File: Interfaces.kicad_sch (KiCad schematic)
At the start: 17 parts, among them J3 Conn_01x04_MountingPin, J4 Conn_01x05_Pin, J5 Conn_01x05_MountingPin, J6 MSD-11-A, U5 TLV74033PDBVR

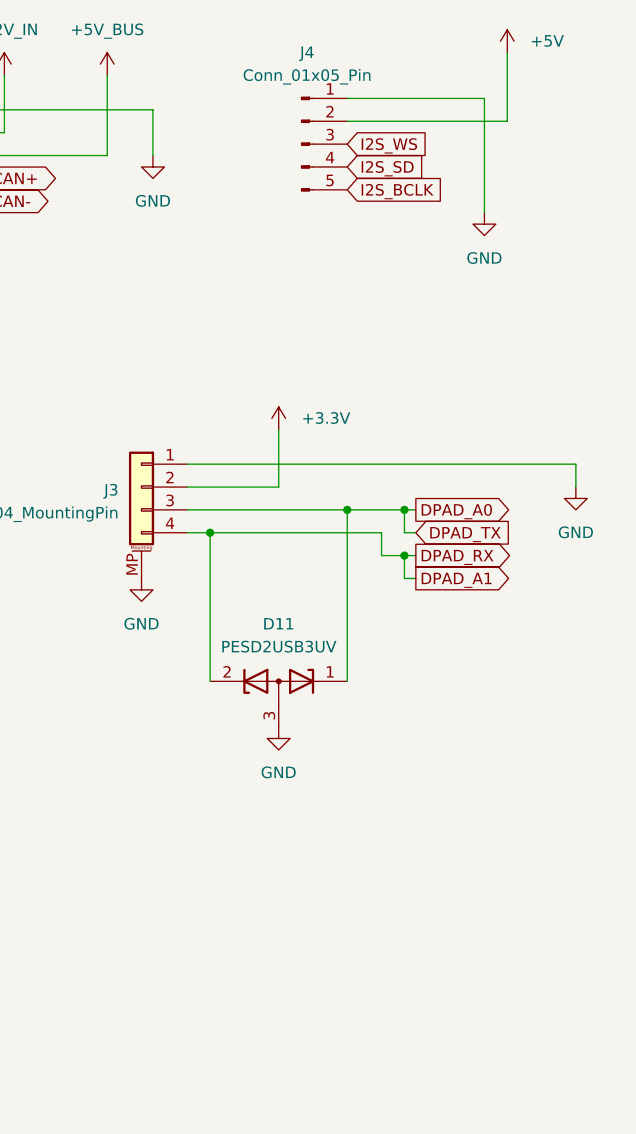
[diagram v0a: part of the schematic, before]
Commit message: r1 final (see changelog.md)
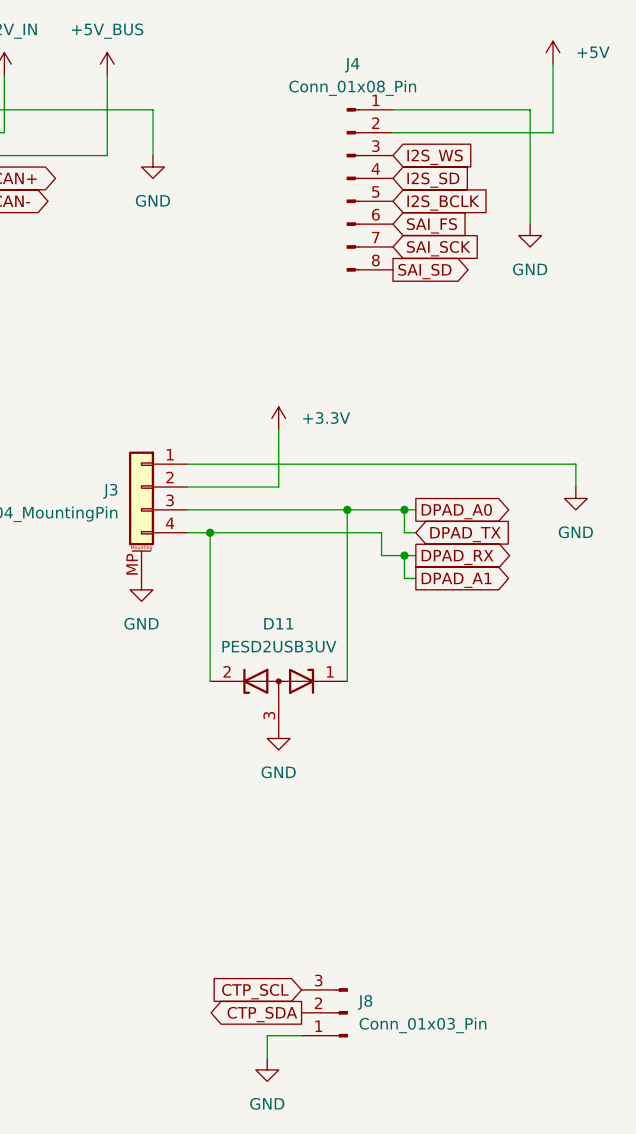
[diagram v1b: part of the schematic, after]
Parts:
- removed J4: Conn_01x05_Pin, Connector_PinHeader_2.54mm:PinHeader_1x05_P2.54mm_Vertical, symbol Connector:Conn_01x05_Pin
- added J4: Conn_01x08_Pin, Connector_PinHeader_2.54mm:PinHeader_1x08_P2.54mm_Vertical, symbol Connector:Conn_01x08_Pin
- added J8: Conn_01x03_Pin, Connector_PinHeader_2.54mm:PinHeader_1x03_P2.54mm_Vertical, symbol Connector:Conn_01x03_Pin
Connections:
- net +5V: now also J4.2 (Pin_2)
- net GND: now also J4.1 (Pin_1), J8.1 (Pin_1)
- net I2S_BCLK: now also J4.5 (Pin_5)
- net I2S_SD: now also J4.4 (Pin_4)
- net I2S_WS: now also J4.3 (Pin_3)
- new net CTP_SCL: J8.3 (Pin_3)
- new net CTP_SDA: J8.2 (Pin_2)
- new net SAI_FS: J4.6 (Pin_6)
- new net SAI_SCK: J4.7 (Pin_7)
- new net SAI_SD: J4.8 (Pin_8)
